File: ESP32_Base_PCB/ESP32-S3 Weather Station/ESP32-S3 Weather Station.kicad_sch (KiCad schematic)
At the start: 96 parts, among them IC1 XL7005A, IC2 XL7005A, J1 USB_C_Receptacle_USB2.0_16P, Q1 Si2306, Q2 CSD19505, Q3 CSD19505, Q4 CSD19505, SW1 PTS810_SJM_250_SMTR_LFS, SW2 PTS810_SJM_250_SMTR_LFS, U1 AMS1117-3.3, U2 ESP32-S3-WROOM-2, U3 ADS1015IDGS, U4 ACS712ELCTR30AT, U6 AMS1117-5.0, U7 IR2104

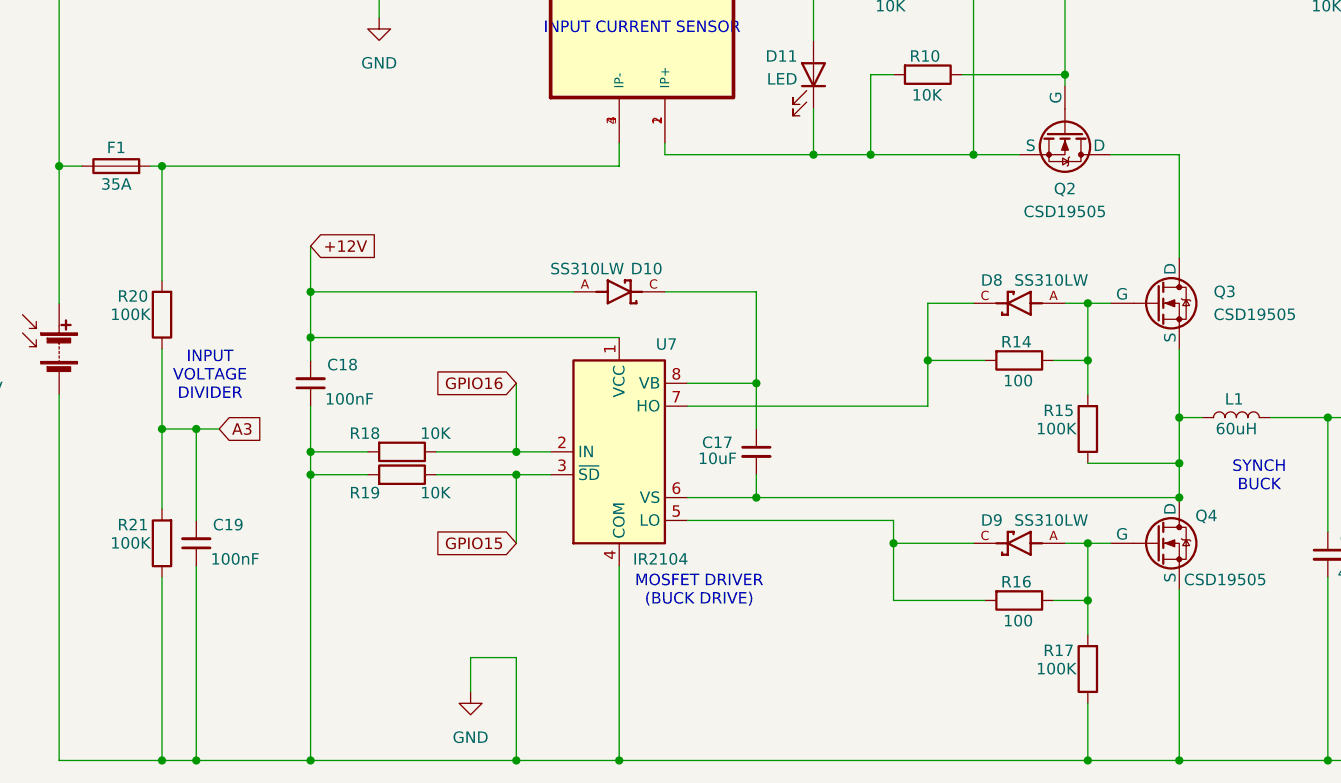
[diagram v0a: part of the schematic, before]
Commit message: more changes
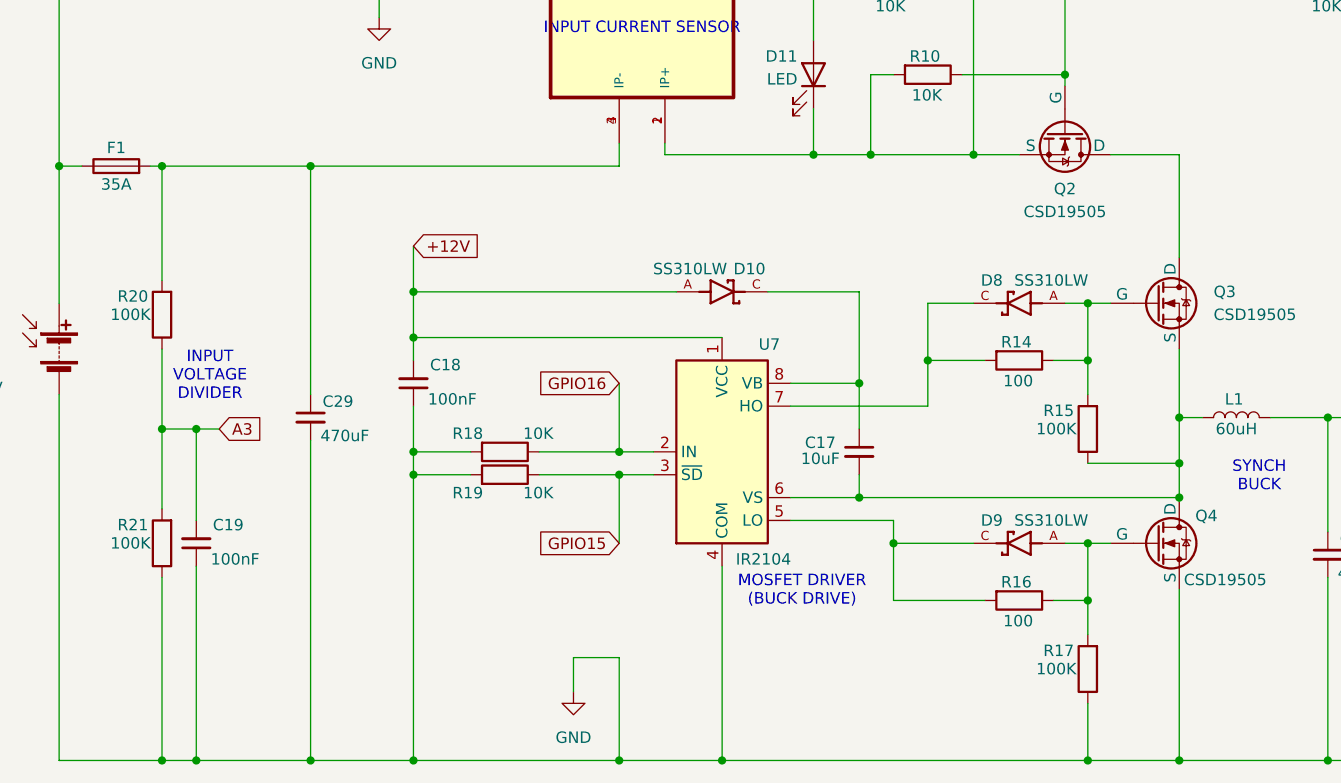
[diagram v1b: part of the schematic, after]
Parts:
- added C29: 470uF, Capacitor_THT:CP_Radial_D16.0mm_P7.50mm, symbol Device:C_Small
- C26: footprint Capacitor_SMD:C_0805_2012Metric_Pad1.18x1.45mm_HandSolder -> Capacitor_THT:CP_Radial_D16.0mm_P7.50mm
- D10, D12, D13, D8, D9: footprint SS310LW:SODFL3718X102N -> (none)
- D11: footprint (none) -> LED_SMD:LED_0805_2012Metric_Pad1.15x1.40mm_HandSolder
- F1, F2: footprint (none) -> Fuse:Fuseholder_Keystone_3555-2
- L1: footprint (none) -> Inductor_THT:L_Toroid_Vertical_L21.6mm_W11.4mm_P7.62mm_Pulse_KM-3
- L2, L3: footprint (none) -> B82442T1104K050:INDM5650X530N
- PS1: footprint CONV_TBA_1-1212 -> (none)
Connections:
- net GND: now also C29.2
- net at F1.2, R20.2, U4.3 (IP-)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: now also C29.1
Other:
- moved on the sheet: C17, C18, D10, R18, R19, U7
